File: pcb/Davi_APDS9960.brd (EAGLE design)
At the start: 77.5 x 100 mm, 11 parts, among them IC1 MEGA8-P, IC2 L293D

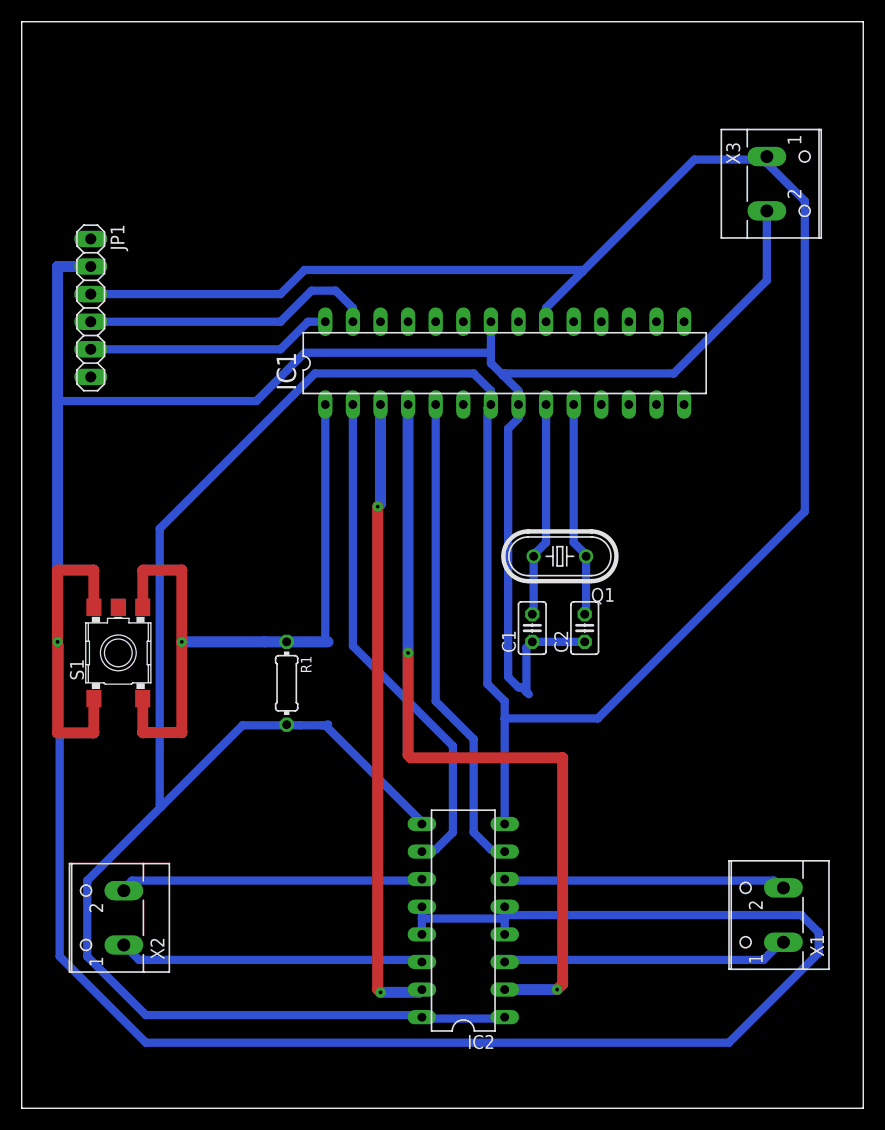
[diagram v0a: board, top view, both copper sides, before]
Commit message: Add files via upload
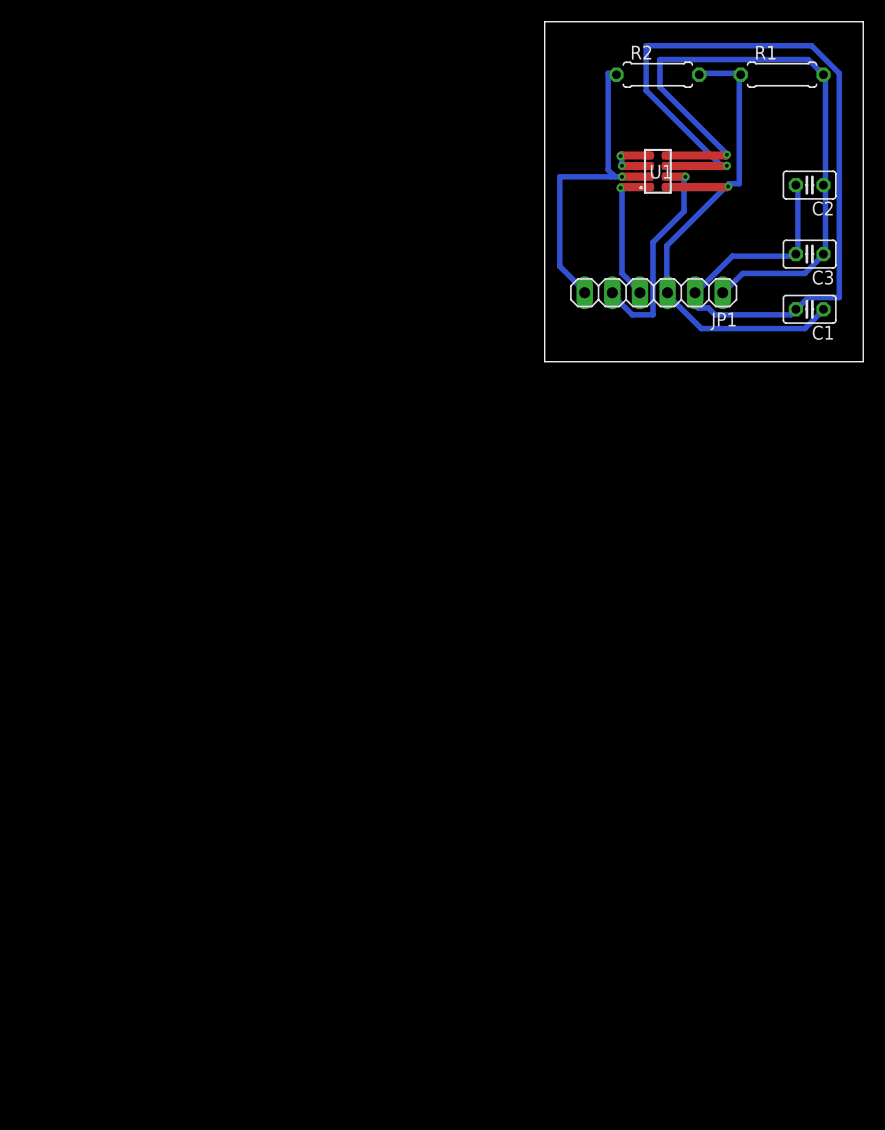
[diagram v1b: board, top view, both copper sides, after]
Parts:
- removed IC1: MEGA8-P, atmel:DIL28-3
- removed IC2: L293D, st-microelectronics:DIL16
- removed Q1: (no value), crystal:HC49U-V
- removed S1: SKHMPSE010, switch:SKHMPXE010
- removed X1, X2, X3: (no value), con-wago-500:W237-102
- added C3: 100uF, rcl:C025-025X050
- added R2: 10k, rcl:0207/7
- added U1: APDS-9960, APDS-9960:APDS-9950
- R1: value (none) -> 10k; device rcl:0204/7 -> rcl:0207/7
- moved R1 72.2 mm to (152.5, 95.1), turned to 0 degrees
- moved JP1 51.8 mm to (140.7, 75.1), turned to 180 degrees
- moved C2 45.7 mm to (155.1, 85.0), turned to 180 degrees
- moved C1 38.9 mm to (155.1, 73.5), turned to 180 degrees
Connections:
- removed net +5V: IC1.20, IC1.7, IC2.1, IC2.16, IC2.8, IC2.9, JP1.3, R1.2, X3.1
- removed net INT: JP1.6
- removed net N$10: IC1.3, IC2.15
- removed net N$11: IC1.2, IC2.10
- removed net N$3: C2.2, IC1.10, Q1.1
- removed net N$5: IC2.6, X1.2
- removed net N$6: IC2.14, X2.1
- removed net N$9: IC1.5, IC2.7
- removed net SCL: IC1.28, JP1.5
- removed net SDA: IC1.27, JP1.4
- removed net VL: JP1.1
- new net VCC: C1.1, JP1.3, R1.1, R2.2, U1.8
- net GND: now also C1.2, C2.2, C3.2, U1.6; no longer C1.1, C2.1, IC1.22, IC1.8, IC2.12, IC2.13, IC2.4, IC2.5, S1.1, S1.2, X3.2
- net N$1: now also U1.3, U1.4; no longer IC1.1, R1.1, S1.3, S1.4
- net N$2: now also C2.1, C3.1, JP1.1, R1.2, U1.5; no longer C1.2, IC1.9, Q1.2
- net N$4: now also JP1.6, R2.1, U1.2; no longer IC2.3, X1.1
- net N$7: now also JP1.4, U1.1; no longer IC2.11, X2.2
- net N$8: now also JP1.5, U1.7; no longer IC1.4, IC2.2
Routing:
- net +5V: track 335.9 -> 0.00 mm
- net GND: track 337.9 -> 92.4 mm
- net N$1: track 66.2 -> 6.38 mm, vias 1 -> 2
- net N$10: track 58.2 -> 0.00 mm, vias 2 -> 0
- net N$8: track 73.0 -> 20.6 mm, vias 2 -> 1
- net VCC: track 0.00 -> 49.8 mm, vias 0 -> 1
- net N$11: track 46.9 -> 0.00 mm
- net N$9: track 44.5 -> 0.00 mm
- net N$2: track 19.9 -> 60.2 mm, vias 0 -> 1
- net N$6: track 28.2 -> 0.00 mm
- net SDA: track 27.2 -> 0.00 mm
- net N$5: track 26.0 -> 0.00 mm
- net SCL: track 22.6 -> 0.00 mm
- net N$3: track 19.9 -> 0.00 mm
- net N$7: track 28.0 -> 13.1 mm, vias 0 -> 1
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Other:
- board size 77.5 x 100 mm -> 29.3 x 31.3 mm
